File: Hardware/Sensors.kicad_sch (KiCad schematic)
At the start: 5 parts, among them J7 Conn_Coaxial, U16 MAX-M10S-00B, U4 BMP581, U5 BMM350, U6 BMI088

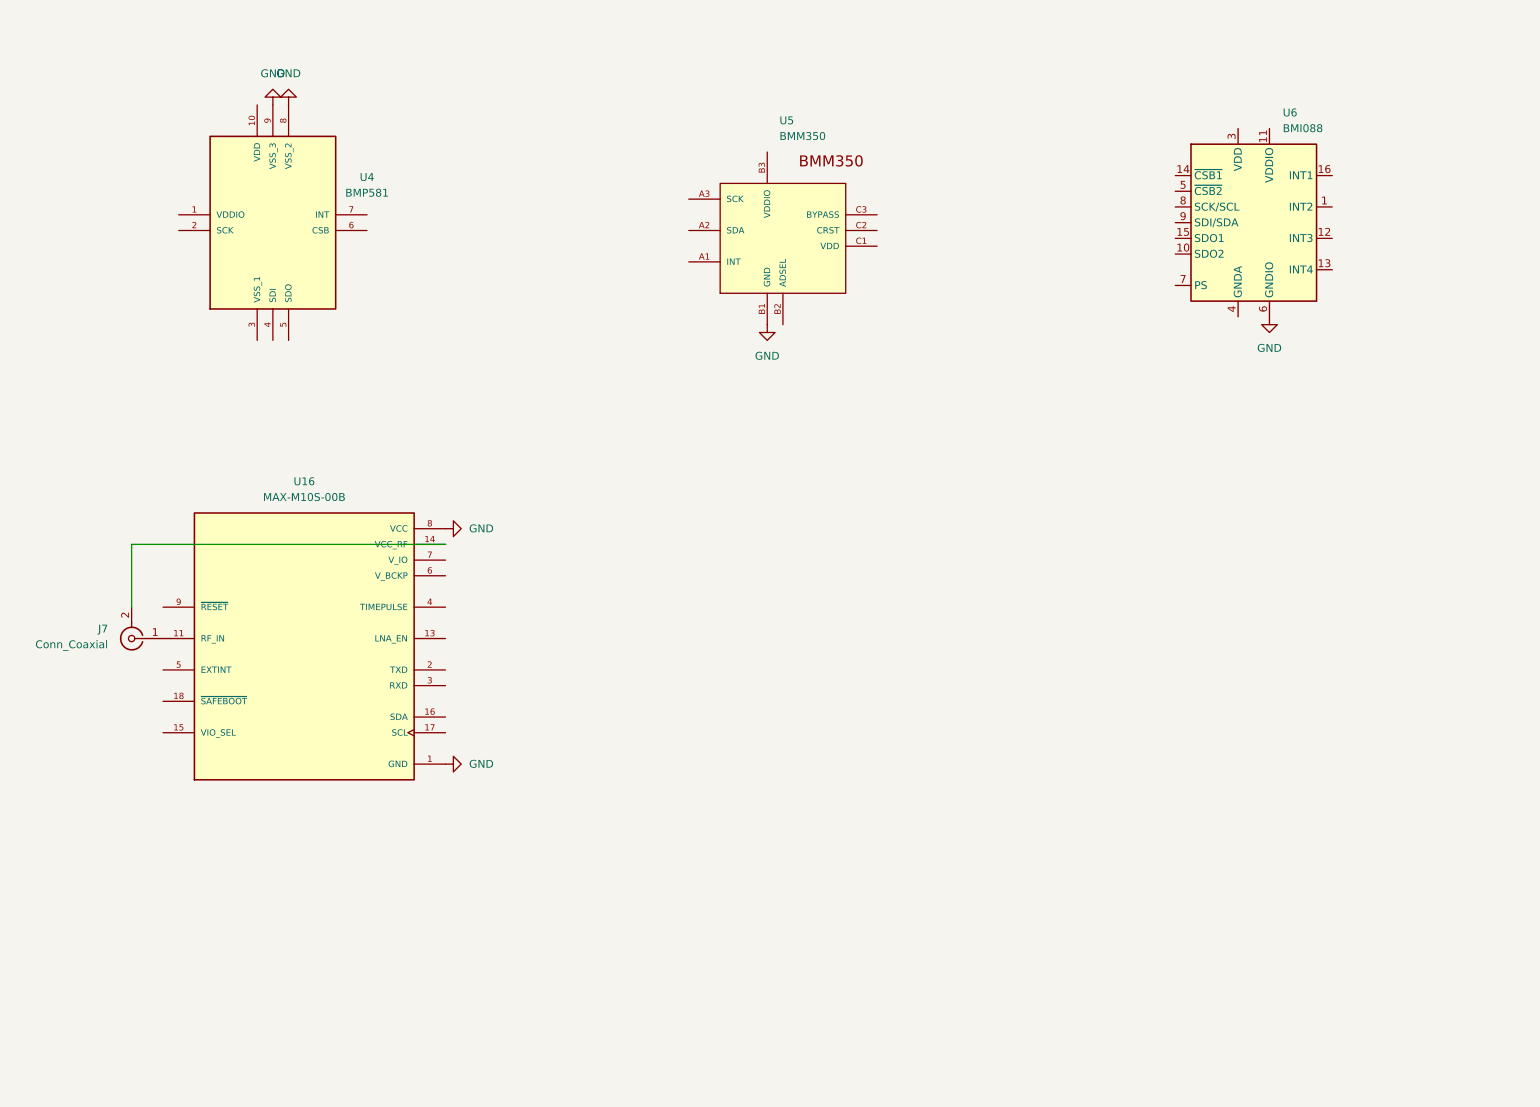
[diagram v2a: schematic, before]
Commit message: 12-March update
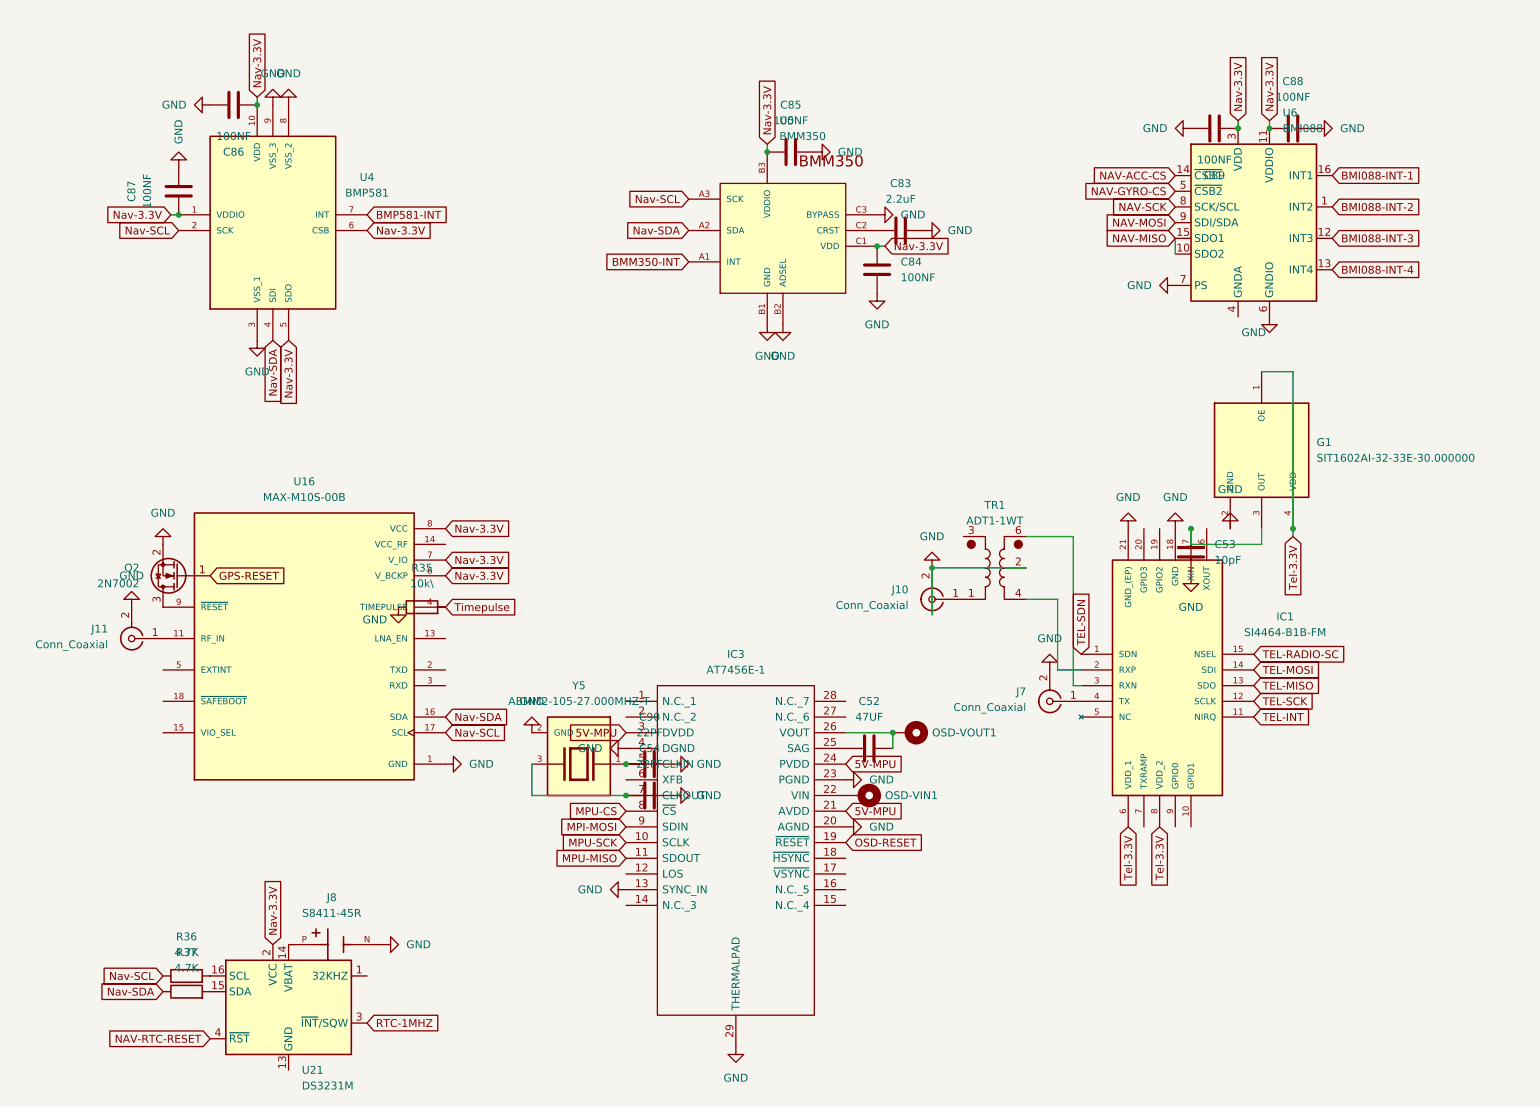
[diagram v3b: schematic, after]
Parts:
- added C52: 47UF, Capacitor_SMD:C_0402_1005Metric, symbol Device:C
- added C53: 10pF, Capacitor_SMD:C_0201_0603Metric, symbol Device:C
- added C54, C90: 22PF, symbol Device:C
- added C83: 2.2uF, Capacitor_SMD:C_0201_0603Metric, symbol Device:C
- added C84, C85, C86, C87, C88, C89: 100NF, Capacitor_SMD:C_0201_0603Metric, symbol Device:C
- added G1: SIT1602AI-32-33E-30.000000, SIT1602AI-32-33E-30.000000:OSC_SIT1602AI-32-33E-30.000000, symbol SIT1602AI-32-33E-30.000000:SIT1602AI-32-33E-30.000000
- added IC1: SI4464-B1B-FM, SI4464-B1B-FM:QFN50P400X400X90-21N, symbol SI4464-B1B-FM:SI4464-B1B-FM
- added IC3: AT7456E-1, AT7456E:SOP65P640X120-29N, symbol Display_Graphic:AT7456E-1
- added J10, J11: Conn_Coaxial, Connector_Coaxial:SMA_Amphenol_901-143_Horizontal, symbol Connector:Conn_Coaxial
- added J8: S8411-45R, S8411-45R:HARWIN_S8411-45R, symbol S8411-45R:S8411-45R
- added OSD-VIN1, OSD-VOUT1: Solderpad, TestPoint:TestPoint_Pad_1.5x1.5mm, symbol Mechanical:Solderpad
- added Q2: 2N7002, Package_TO_SOT_SMD:SOT-23, symbol Transistor_FET:2N7002
- added R35: 10k\, Resistor_SMD:R_0201_0603Metric, symbol Device:R
- added R36, R37: 4.7K, Resistor_SMD:R_0201_0603Metric, symbol Device:R
- added TR1: ADT1-1WT, RF_Mini-Circuits:Mini-Circuits_CD542_H2.84mm, symbol Transformer:ADT1-1WT
- added U21: DS3231M, Package_SO:SOIC-16W_7.5x10.3mm_P1.27mm, symbol Timer_RTC:DS3231M
- added Y5: ABMM2-105-27.000MHZ-T, ABMM2-105-27.000MHZ-T:XTAL_ABMM2-105-27.000MHZ-T, symbol ABMM2-105-27.000MHZ-T:ABMM2-105-27.000MHZ-T
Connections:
- net GND: now also J7.2 (Ext), U4.3 (VSS_1), U5.B2 (ADSEL), U5.C3 (BYPASS), U6.7 (PS), C53.2, C54.2, C83.2, C84.2, C85.2, C86.2, C87.2, C88.2, C89.2, C90.2, G1.2 (GND), IC1.18 (GND), IC1.21 (GND_(EP)), IC3.13 (SYNC_IN), IC3.20 (AGND), IC3.23 (PGND), IC3.29 (THERMALPAD), IC3.4 (DGND), J10.2 (Ext), J11.2 (Ext), J8.N, Q2.2 (S), R35.1, TR1.2, Y5.2 (GND), Y5.4 (GND); no longer U16.8 (VCC)
- net BMI088-INT-2: now reaches U6.1 (INT2)
- net NAV-MISO: now reaches U6.10 (SDO2)
- net NAV-MISO: now also U6.15 (SDO1)
- net Nav-3.3V: now reaches U6.11 (VDDIO)
- net Nav-3.3V: now also U16.6 (V_BCKP), U16.7 (V_IO), U16.8 (VCC), U4.1 (VDDIO), U4.10 (VDD), U4.5 (SDO), U4.6 (CSB), U5.B3 (VDDIO), U5.C1 (VDD), U6.3 (VDD), C84.1, C85.1, C86.1, C87.1, C88.1, C89.1, U21.2 (VCC)
- net BMI088-INT-3: now reaches U6.12 (INT3)
- net BMI088-INT-4: now reaches U6.13 (INT4)
- net NAV-ACC-CS: now reaches U6.14 (~{CSB1})
- net BMI088-INT-1: now reaches U6.16 (INT1)
- net NAV-GYRO-CS: now reaches U6.5 (~{CSB2})
- net NAV-SCK: now reaches U6.8 (SCK/SCL)
- net NAV-MOSI: now reaches U6.9 (SDI/SDA)
- net at J7.1 (In): now also IC1.4 (TX); no longer U16.11 (RF_IN)
- net at U16.14 (VCC_RF): no longer J7.2 (Ext)
- net Nav-SCL: now reaches U4.2 (SCK)
- net Nav-SCL: now also U16.17 (SCL), U5.A3 (SCK), R36.1
- net Nav-SDA: now reaches U4.4 (SDI)
- net Nav-SDA: now also U16.16 (SDA), U5.A2 (SDA), R37.1
- net BMP581-INT: now reaches U4.7 (INT)
- net BMM350-INT: now reaches U5.A1 (INT)
- net at U5.C2 (CRST): now also C83.1
- net Timepulse: now reaches U16.4 (TIMEPULSE)
- net Timepulse: now also R35.2
- net at U16.9 (~{RESET}): now also Q2.3 (D)
- new net: C52.1, IC3.25 (SAG)
- new net: C52.2, IC3.26 (VOUT), OSD-VOUT1.1
- new net: C54.1, IC3.7 (CLKOUT), Y5.3
- new net: U21.10 (GND), U21.11 (GND), U21.12 (GND), U21.13 (GND), U21.5 (GND), U21.6 (GND), U21.7 (GND), U21.8 (GND), U21.9 (GND)
- new net: J8.P, U21.14 (VBAT)
- new net: R37.2, U21.15 (SDA)
- new net: R36.2, U21.16 (SCL)
- new net: C53.1, G1.3 (OUT), IC1.17 (XIN)
- new net: C90.1, IC3.5 (CLKIN), Y5.1
- new net: IC3.22 (VIN), OSD-VIN1.1
- new net: IC1.2 (RXP), TR1.4
- new net: IC1.3 (RXN), TR1.6
- new net: J10.1 (In), TR1.1
- new net: J11.1 (In), U16.11 (RF_IN)
- new net 5V-MPU: IC3.21 (AVDD), IC3.24 (PVDD), IC3.3 (DVDD)
- new net GPS-RESET: Q2.1 (G)
- new net MPI-MOSI: IC3.9 (SDIN)
- new net MPU-CS: IC3.8 (~{CS})
- new net MPU-MISO: IC3.11 (SDOUT)
- new net MPU-SCK: IC3.10 (SCLK)
- new net NAV-RTC-RESET: U21.4 (~{RST})
- new net OSD-RESET: IC3.19 (~{RESET})
- new net RTC-1MHZ: U21.3 (~{INT}/SQW)
- new net TEL-INT: IC1.11 (NIRQ)
- new net TEL-MISO: IC1.13 (SDO)
- new net TEL-MOSI: IC1.14 (SDI)
- new net TEL-RADIO-SC: IC1.15 (NSEL)
- new net TEL-SCK: IC1.12 (SCLK)
- new net TEL-SDN: IC1.1 (SDN)
- new net Tel-3.3V: G1.1 (OE), G1.4 (VDD), IC1.6 (VDD_1), IC1.8 (VDD_2)
